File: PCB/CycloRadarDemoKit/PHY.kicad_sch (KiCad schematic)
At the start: 34 parts, among them J301 TMJD0012BENL, U301 IP101GRI, Y301 25MHz

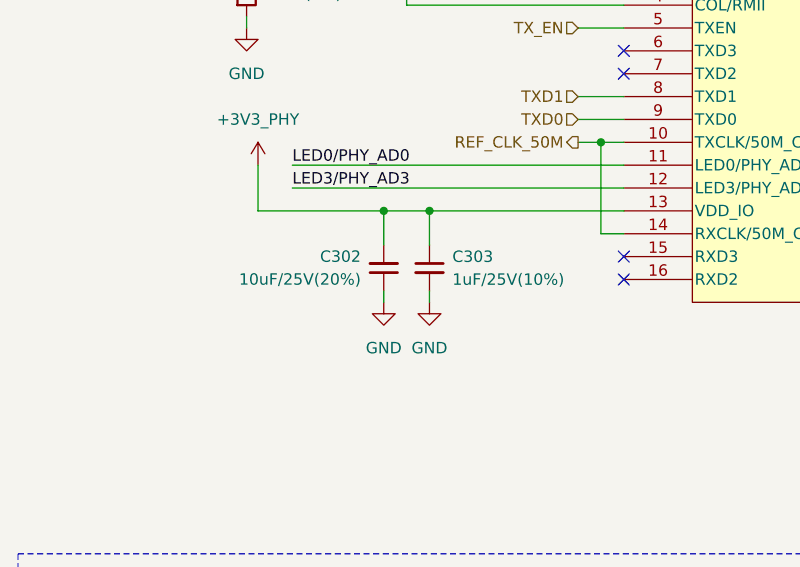
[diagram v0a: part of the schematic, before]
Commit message: start of repair after review
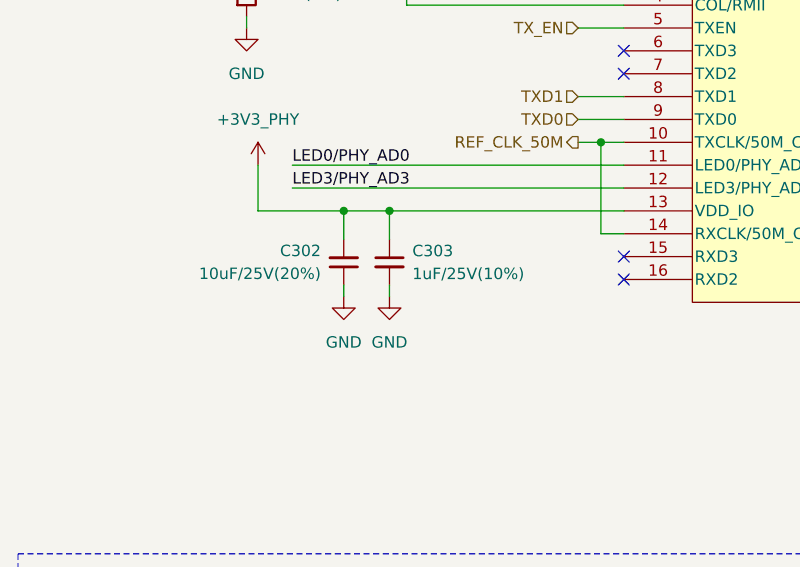
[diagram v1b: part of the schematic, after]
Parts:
- R312: now left out of the parts list
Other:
- moved on the sheet: C302, C303
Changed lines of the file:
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@@
   (junction (at 273.05 140.97) (diameter 0) (color 0 0 0 0)
   )
-  (junction (at 69.85 80.01) (diameter 0) (color 0 0 0 0)
-  )
-  (junction (at 64.77 80.01) (diameter 0) (color 0 0 0 0)
-  )
   (junction (at 205.74 49.53) (diameter 0) (color 0 0 0 0)
   )
@@
   (junction (at 49.53 163.83) (diameter 0) (color 0 0 0 0)
   )
+  (junction (at 60.325 80.01) (diameter 0) (color 0 0 0 0)
+  )
   (junction (at 97.155 167.005) (diameter 0) (color 0 0 0 0)
   )
@@
   )
   (junction (at 182.88 92.71) (diameter 0) (color 0 0 0 0)
+  )
+  (junction (at 65.405 80.01) (diameter 0) (color 0 0 0 0)
   )
   (junction (at 81.28 49.53) (diameter 0) (color 0 0 0 0)
@@
     (stroke (width 0) (type default))
   )
-  (wire (pts (xy 69.85 80.01) (xy 91.44 80.01))
-    (stroke (width 0) (type default))
-  )
   (wire (pts (xy 123.19 31.75) (xy 129.54 31.75))
     (stroke (width 0) (type default))
@@
     (stroke (width 0) (type default))
   )
-  (wire (pts (xy 64.77 88.9) (xy 64.77 90.17))
+  (wire (pts (xy 60.325 88.265) (xy 60.325 89.535))
     (stroke (width 0) (type default))
   )
@@
     (stroke (width 0) (type default))
   )
-  (wire (pts (xy 64.77 80.01) (xy 64.77 83.82))
+  (wire (pts (xy 60.325 80.01) (xy 60.325 83.185))
     (stroke (width 0) (type default))
   )
@@
     (stroke (width 0) (type default))
   )
-  (wire (pts (xy 64.77 80.01) (xy 69.85 80.01))
+  (wire (pts (xy 60.325 80.01) (xy 65.405 80.01))
     (stroke (width 0) (type default))
   )
@@
     (stroke (width 0) (type default))
   )
+  (wire (pts (xy 65.405 80.01) (xy 91.44 80.01))
+    (stroke (width 0) (type default))
+  )
   (wire (pts (xy 49.53 157.48) (xy 49.53 154.94))
     (stroke (width 0) (type default))
@@
     (stroke (width 0) (type default))
   )
-  (wire (pts (xy 69.85 80.01) (xy 69.85 83.82))
+  (wire (pts (xy 65.405 80.01) (xy 65.405 83.185))
     (stroke (width 0) (type default))
   )
@@
     (stroke (width 0) (type default))
   )
-  (wire (pts (xy 50.8 80.01) (xy 64.77 80.01))
+  (wire (pts (xy 50.8 80.01) (xy 60.325 80.01))
     (stroke (width 0) (type default))
   )
@@
     (stroke (width 0) (type default))
   )
-  (wire (pts (xy 69.85 88.9) (xy 69.85 90.17))
+  (wire (pts (xy 65.405 88.265) (xy 65.405 89.535))
     (stroke (width 0) (type default))
   )
@@
     )
   )
-  (symbol (lib_id "Device:C_Small") (at 64.77 86.36 0) (mirror x) (unit 1)
+  (symbol (lib_id "Device:C_Small") (at 60.325 85.725 0) (mirror x) (unit 1)
     (in_bom yes) (on_board yes) (dnp no)
-    (property "Reference" "C302" (at 62.23 85.0836 0)
+    (property "Reference" "C302" (at 57.785 84.4486 0)
       (effects (font (size 1.27 1.27)) (justify right))
     )
-    (property "Value" "10uF/25V(20%)" (at 62.23 87.6236 0)
+    (property "Value" "10uF/25V(20%)" (at 57.785 86.9886 0)
       (effects (font (size 1.27 1.27)) (justify right))
     )
-    (property "Footprint" "Capacitor_SMD:C_0603_1608Metric" (at 64.77 86.36 0)
-      (effects (font (size 1.27 1.27)) hide)
-    )
-    (property "Datasheet" "~" (at 64.77 86.36 0)
-      (effects (font (size 1.27 1.27)) hide)
-    )
-    (property "LCSC" "C96446" (at 64.77 86.36 0)
+    (property "Footprint" "Capacitor_SMD:C_0603_1608Metric" (at 60.325 85.725 0)
+      (effects (font (size 1.27 1.27)) hide)
+    )
+    (property "Datasheet" "~" (at 60.325 85.725 0)
+      (effects (font (size 1.27 1.27)) hide)
+    )
+    (property "LCSC" "C96446" (at 60.325 85.725 0)
       (effects (font (size 1.27 1.27)) hide)
     )
@@
     )
   )
-  (symbol (lib_id "Device:C_Small") (at 69.85 86.36 0) (unit 1)
+  (symbol (lib_id "Device:C_Small") (at 65.405 85.725 0) (unit 1)
     (in_bom yes) (on_board yes) (dnp no)
-    (property "Reference" "C303" (at 72.39 85.0963 0)
-      (effects (font (size 1.27 1.27)) (justify left))
-    )
-    (property "Value" "1uF/25V(10%)" (at 72.39 87.6363 0)
-      (effects (font (size 1.27 1.27)) (justify left))
-    )
-    (property "Footprint" "Capacitor_SMD:C_0402_1005Metric" (at 69.85 86.36 0)
-      (effects (font (size 1.27 1.27)) hide)
-    )
-    (property "Datasheet" "~" (at 69.85 86.36 0)
-      (effects (font (size 1.27 1.27)) hide)
-    )
-    (property "LCSC" "C52923" (at 69.85 86.36 0)
+    (property "Reference" "C303" (at 67.945 84.4613 0)
+      (effects (font (size 1.27 1.27)) (justify left))
+    )
+    (property "Value" "1uF/25V(10%)" (at 67.945 87.0013 0)
+      (effects (font (size 1.27 1.27)) (justify left))
+    )
+    (property "Footprint" "Capacitor_SMD:C_0402_1005Metric" (at 65.405 85.725 0)
+      (effects (font (size 1.27 1.27)) hide)
+    )
+    (property "Datasheet" "~" (at 65.405 85.725 0)
+      (effects (font (size 1.27 1.27)) hide)
+    )
+    (property "LCSC" "C52923" (at 65.405 85.725 0)
       (effects (font (size 1.27 1.27)) hide)
     )
@@
     )
   )
-  (symbol (lib_id "power:GND") (at 69.85 90.17 0) (unit 1)
-    (in_bom yes) (on_board yes) (dnp no) (fields_autoplaced)
-    (property "Reference" "#PWR0313" (at 69.85 96.52 0)
-      (effects (font (size 1.27 1.27)) hide)
-    )
-    (property "Value" "GND" (at 69.85 95.25 0)
-      (effects (font (size 1.27 1.27)))
-    )
-    (property "Footprint" "" (at 69.85 90.17 0)
-      (effects (font (size 1.27 1.27)) hide)
-    )
-    (property "Datasheet" "" (at 69.85 90.17 0)
+  (symbol (lib_id "power:GND") (at 65.405 89.535 0) (unit 1)
+    (in_bom yes) (on_board yes) (dnp no) (fields_autoplaced)
+    (property "Reference" "#PWR0313" (at 65.405 95.885 0)
+      (effects (font (size 1.27 1.27)) hide)
+    )
+    (property "Value" "GND" (at 65.405 94.615 0)
+      (effects (font (size 1.27 1.27)))
+    )
+    (property "Footprint" "" (at 65.405 89.535 0)
+      (effects (font (size 1.27 1.27)) hide)
+    )
+    (property "Datasheet" "" (at 65.405 89.535 0)
       (effects (font (size 1.27 1.27)) hide)
     )
@@
   )
   (symbol (lib_id "Device:R") (at 231.14 140.97 180) (unit 1)
-    (in_bom yes) (on_board yes) (dnp yes) (fields_autoplaced)
+    (in_bom no) (on_board yes) (dnp yes) (fields_autoplaced)
     (property "Reference" "R312" (at 233.045 139.7 0)
       (effects (font (size 1.27 1.27)) (justify right))
@@
     )
   )
-  (symbol (lib_id "power:GND") (at 64.77 90.17 0) (unit 1)
-    (in_bom yes) (on_board yes) (dnp no) (fields_autoplaced)
-    (property "Reference" "#PWR0312" (at 64.77 96.52 0)
-      (effects (font (size 1.27 1.27)) hide)
-    )
-    (property "Value" "GND" (at 64.77 95.25 0)
-      (effects (font (size 1.27 1.27)))
-    )
-    (property "Footprint" "" (at 64.77 90.17 0)
-      (effects (font (size 1.27 1.27)) hide)
-    )
-    (property "Datasheet" "" (at 64.77 90.17 0)
-      (effects (font (size 1.27 1.27)) hide)
-    )
+  (symbol (lib_id "power:GND") (at 60.325 89.535 0) (unit 1)
+    (in_bom yes) (on_board yes) (dnp no) (fields_autoplaced)
+    (property "Reference" "#PWR0312" (at 60.325 95.885 0)
+      (effects (font (size 1.27 1.27)) hide)
+    )
+    (property "Value" "GND" (at 60.325 94.615 0)
+      (effects (font (size 1.27 1.27)))
+    )
+    (property "Footprint" "" (at 60.325 89.535 0)
+      (effects (font (size 1.27 1.27)) hide)
+    )
+    (property "Datasheet" "" (at 60.325 89.535 0)
+      (effects (font (size 1.27 1.27)) hide)
+    )
